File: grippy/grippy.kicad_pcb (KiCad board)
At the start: 2 copper layers, 60.8 x 35.2 mm, 9 parts, among them J1 Conn_01x08_Socket, SW0 SW_SPST, SW1 SW_SPST, SW2 SW_SPST, SW3 SW_SPST, SW4 SW_SPST, SW5 SW_DPDT_x2, U1 esp32s3-supermini

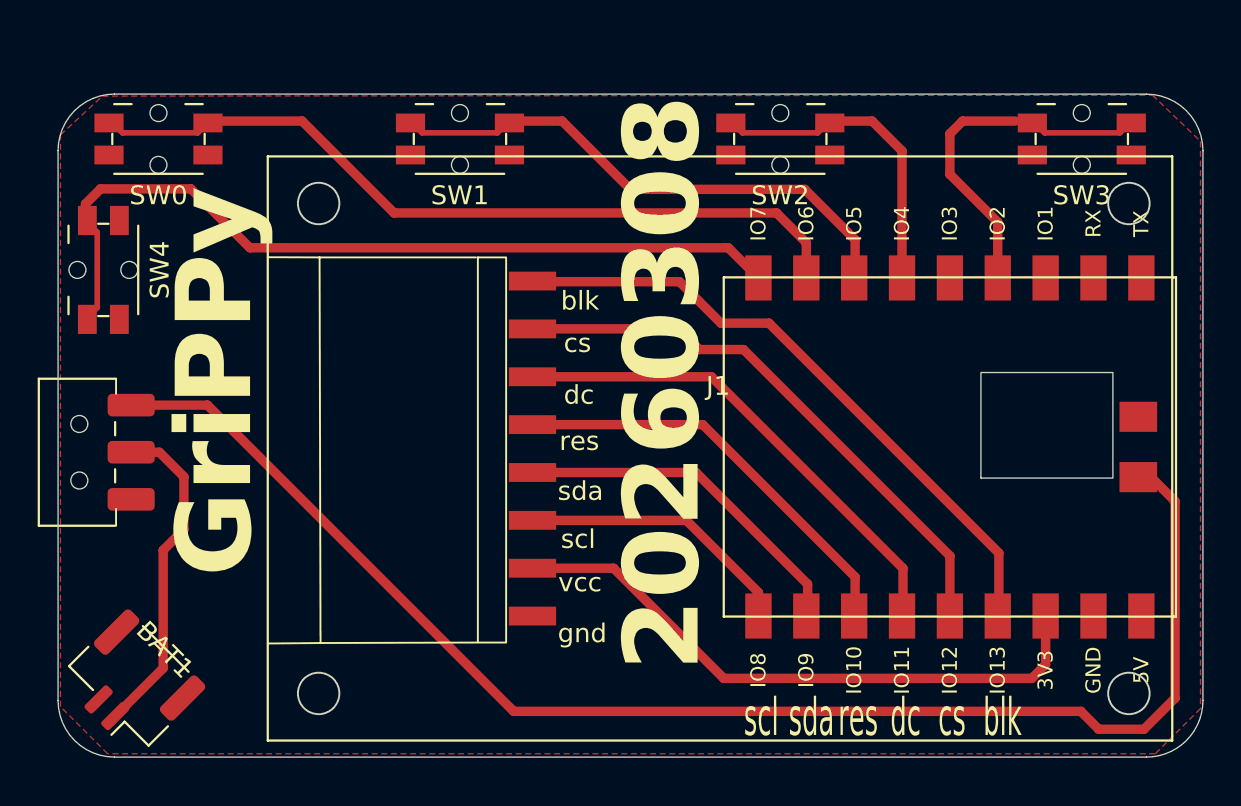
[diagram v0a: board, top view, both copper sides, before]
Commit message: update KiCad/FreeCAD design files, add .gitignore
Add .gitignore to exclude .DS_Store, .FCBak, and backup ZIPs.
Update PCB, STEP, Gerber, and FreeCAD source files to latest local state.

Co-Authored-By: Claude Sonnet 4.6 <noreply@anthropic.com>
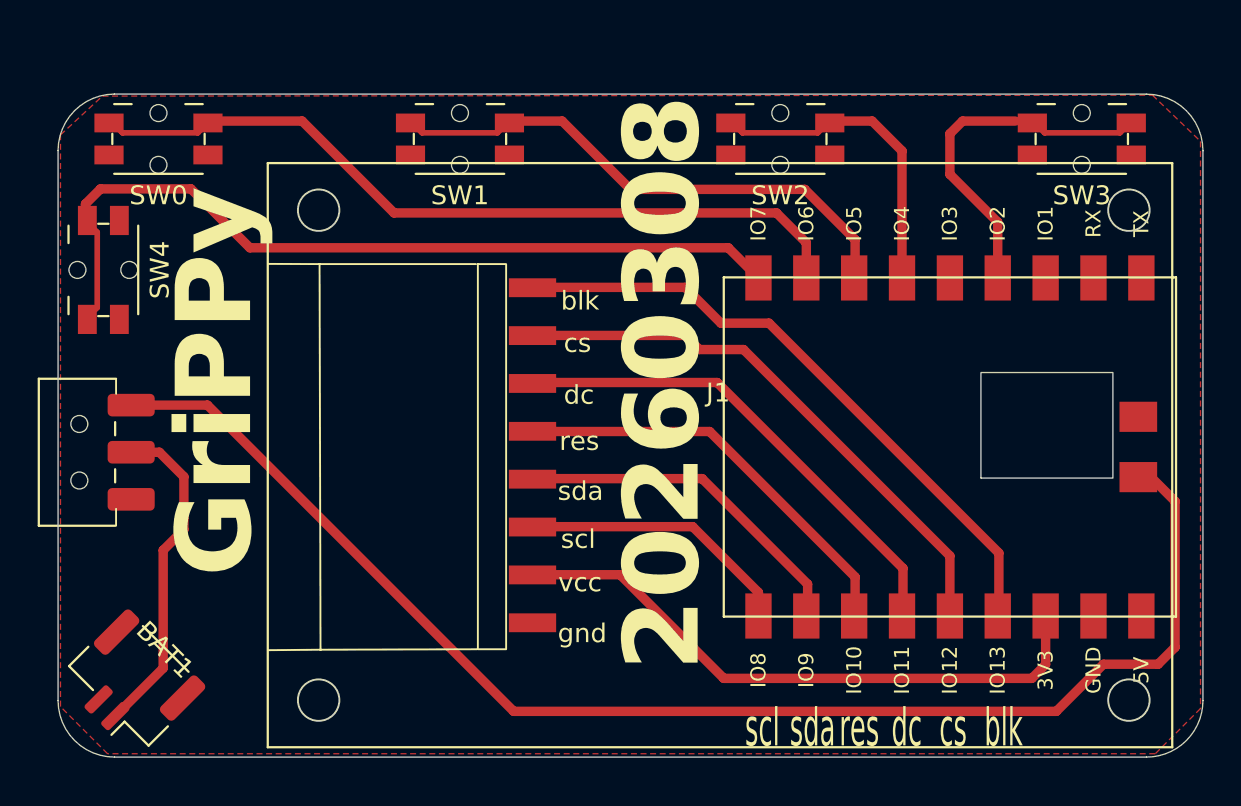
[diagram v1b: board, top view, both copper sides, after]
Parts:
- moved J1 0.36 mm to (212.0, 85.9)
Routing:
- net /RAW: track 76.1 -> 73.8 mm
- net /RES: track 22.8 -> 22.3 mm
